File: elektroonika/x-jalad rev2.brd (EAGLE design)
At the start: 100 x 81 mm, 48 parts, among them Q1 FC-12M

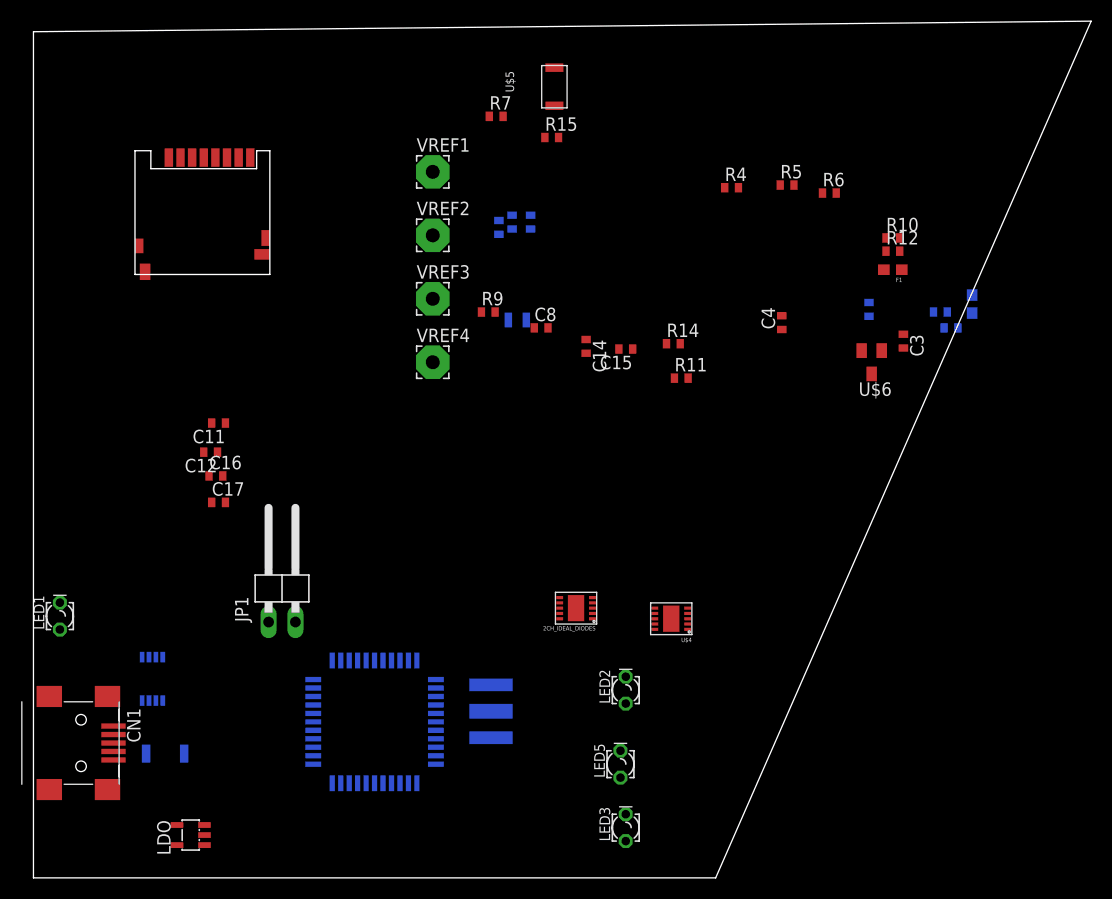
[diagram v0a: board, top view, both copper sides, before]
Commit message: eagle files init
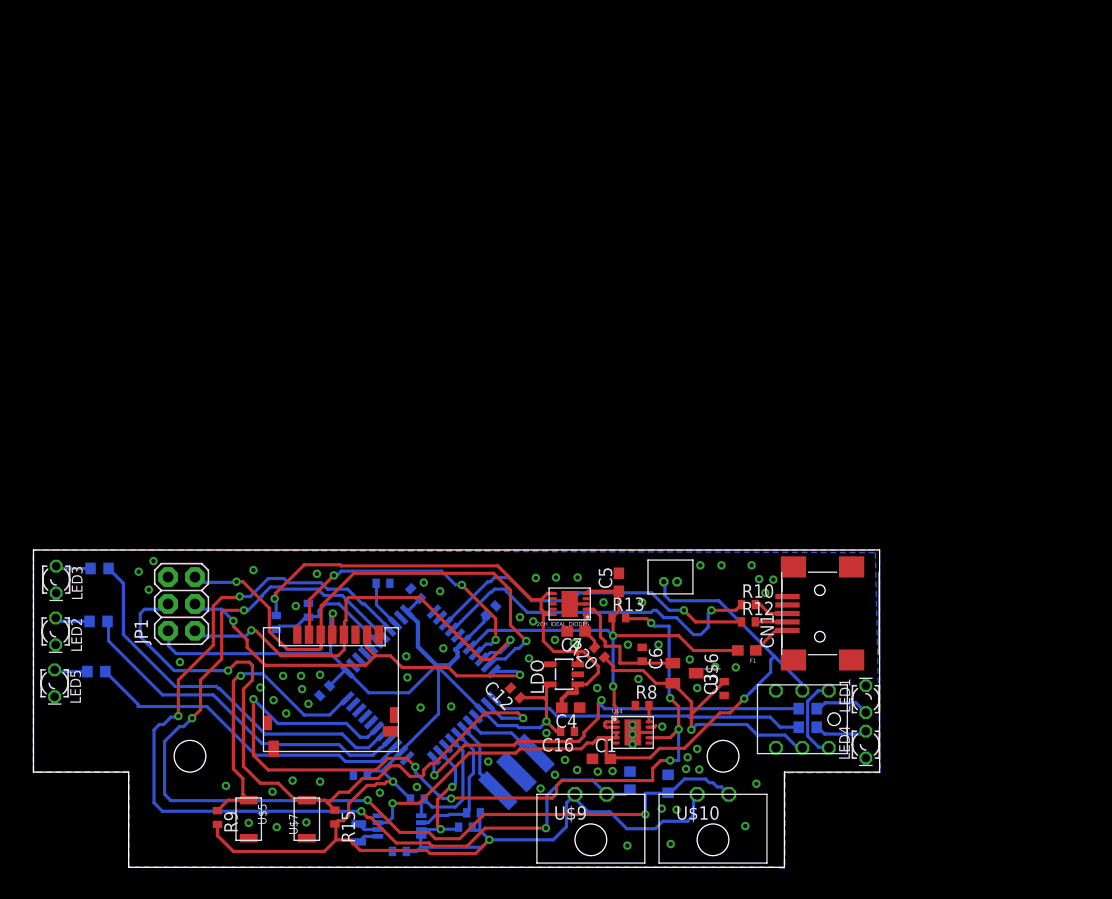
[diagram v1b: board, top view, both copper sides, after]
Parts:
- removed VREF1, VREF2, VREF3, VREF4: (no value), wirepad:3,17/1,3
- added C2, C6: 100nF, eagle-ltspice:C0402
- added C7: 4.7uF, rcl:C0603
- added LED4: (no value), led:LD260
- added R16, R17: 100k, rcl:R0603
- added R18: 1k, rcl:R0603
- added R20: 1k, eagle-ltspice:R0402
- added U$10, U$9: TE_CONNECTIVITY_2-1445055-2, Pressure_sensor_connector:PRESSURE_SENSOR_CONNECTOR
- added U$11: MOLEX-530470210, pwr_connector:SMD_PINHEADER
- added U$8: SPPH410100, start_button:SMD_LATCHING_BUTTON
- C1, C4: device eagle-ltspice:C0402 -> rcl:C0603
- C5: value 4.7 uF -> (none)
- JP1: device pinhead:1X02/90 -> SparkFun:2X03
- R4, R5, R6, R7: device eagle-ltspice:R0402 -> rcl:R0603
- moved R6 77.6 mm to (6.25, 28.2), flipped to the bottom, turned to 180 degrees
- moved R5 77.1 mm to (6.15, 23.2), flipped to the bottom, turned to 180 degrees
- moved LED1 76.6 mm to (78.7, 15.9)
- moved U$5 73.1 mm to (25.9, 2.75)
- moved CN1 72.9 mm to (75.3, 24.0), turned to 90 degrees
- moved R15 67.4 mm to (28.5, 4.75), turned to 270 degrees
- moved R7 64.7 mm to (5.95, 18.5), flipped to the bottom, turned to 180 degrees
- moved LED3 58.7 mm to (2.15, 27.2), turned to 270 degrees
- moved R1 57.5 mm to (40.9, 3.80), turned to 180 degrees
- moved R2 56.0 mm to (41.6, 5.15), turned to 180 degrees
- moved R3 54.6 mm to (36.3, 6.45), turned to 0 degrees
- moved R9 54.2 mm to (17.4, 4.70), turned to 270 degrees
- moved LED2 54.2 mm to (2.10, 22.3), turned to 270 degrees
- moved LED5 54.0 mm to (2.00, 17.4), turned to 270 degrees
- moved Q1 50.8 mm to (30.8, 3.25), turned to 270 degrees
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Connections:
- net NRST1 renamed HWB
- removed net TRGGR: 2CH_IDEAL_DIODES.ENBA, U$6.RST
- new net LED4: R18.2, U$2.12
- new net N$10: 2CH_IDEAL_DIODES.INA, C7.1, R20.2
- new net N$2: C1.2, RTC.VBAT, U$11.P$2, U$4.VBAT, U$4.VBAT2, U$8.P$5
- new net N$7: LED4.A, R18.1
- new net N$8: U$8.P$3, U$8.P$6
- new net N$9: 2CH_IDEAL_DIODES.ENBA, C6.2, U$6.RST
- net +3V3: now also R20.1, U$8.P$2; no longer 2CH_IDEAL_DIODES.INA, C1.2, JP1.2, RTC.VBAT, U$4.VBAT
- net +5V: now also U$2.7
- net GND: now also C2.2, C6.1, C7.2, JP1.6, LED4.K, R16.2, R17.2, U$11.P$1; no longer JP1.1, VREF2.1, VREF4.1
- net LED0: now also R6.2; no longer R7.2
- net LED1: now also R5.2; no longer R6.2
- net LED2: now also R4.2; no longer R5.2
- net LED3: now also R7.2; no longer R4.2
- net MISO: now also JP1.3
- net MOSI: now also JP1.5
- net NRST: now also JP1.4
- net S0_ADC: now also R16.1, U$9.P$2; no longer VREF1.1
- net S1_ADC: now also R17.1, U$10.P$2; no longer VREF3.1
- net SCK: now also JP1.1
- net VCC: now also C2.1, JP1.2, U$10.P$1, U$9.P$1; no longer U$2.7
- net VCC/2: now also LDO.EN
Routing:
- net VCC: track 0.00 -> 170.6 mm, vias 0 -> 4
- net S1_ADC: track 0.00 -> 97.3 mm, vias 0 -> 4
- net S0_ADC: track 0.00 -> 93.1 mm, vias 0 -> 4
- net PB4: track 0.00 -> 85.3 mm, vias 0 -> 7
- net N$2: track 0.00 -> 68.1 mm, vias 0 -> 2
- net NRST: track 0.00 -> 65.0 mm, vias 0 -> 2
- net MOSI: track 0.00 -> 50.2 mm, vias 0 -> 2
- net VCC/2: track 0.00 -> 49.9 mm, vias 0 -> 1
- net +5V: track 0.00 -> 45.3 mm, vias 0 -> 2
- net SCK: track 0.00 -> 43.0 mm, vias 0 -> 2
- net LED2: track 0.00 -> 40.7 mm, vias 0 -> 2
- net MISO: track 0.00 -> 40.0 mm, vias 0 -> 2
- net LED0: track 0.00 -> 36.4 mm
- net LED1: track 0.00 -> 33.5 mm
- net USB_D+: track 0.00 -> 32.9 mm, vias 0 -> 1
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- added copper zone on layer 1, net GND
- added copper zone on layer 16, net GND
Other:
- board size 100 x 81 mm -> 80 x 30 mm
